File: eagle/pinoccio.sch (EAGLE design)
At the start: 48 parts, among them Q1 16MHz, Q2 32.768k, Q4 MOSFET-PCHANNEL, Q5 TRANSISTOR-NPN-DUAL, U1 MCP73831, U2 3.3V, U4 ATMEGA128RFA1, X1 USB-MICROB, Y2 ANTENNA2SMD5

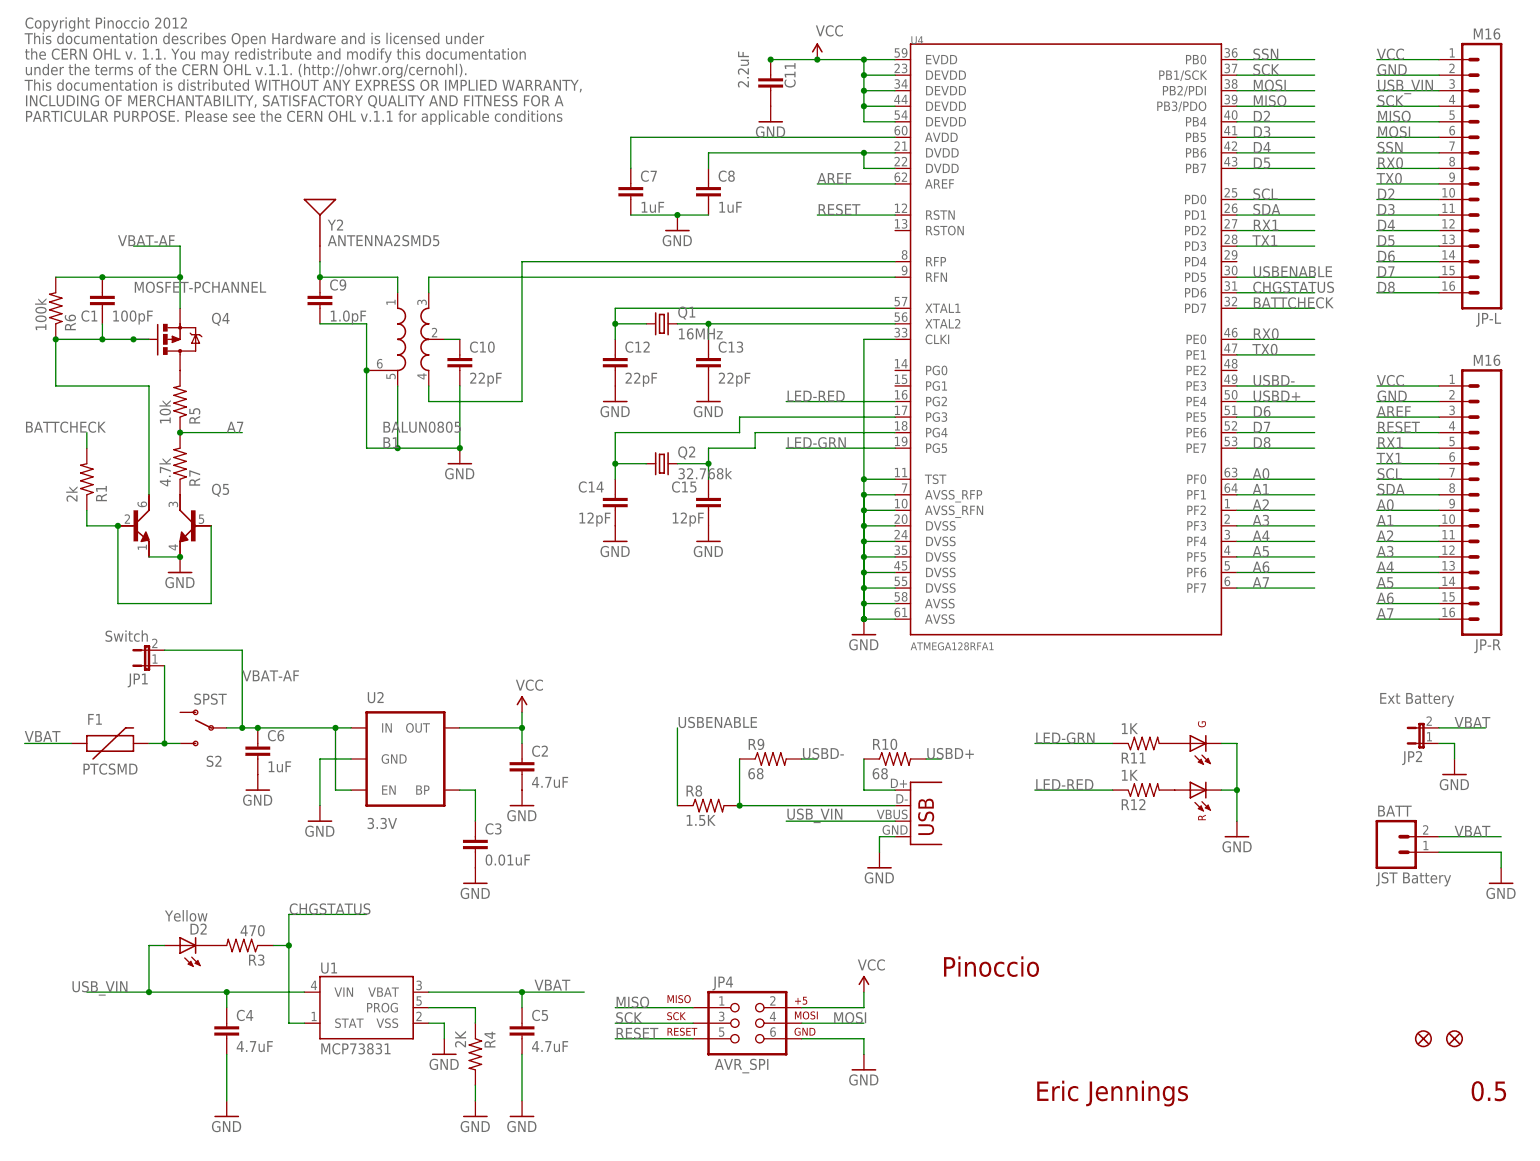
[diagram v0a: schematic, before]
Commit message: Version 0.6
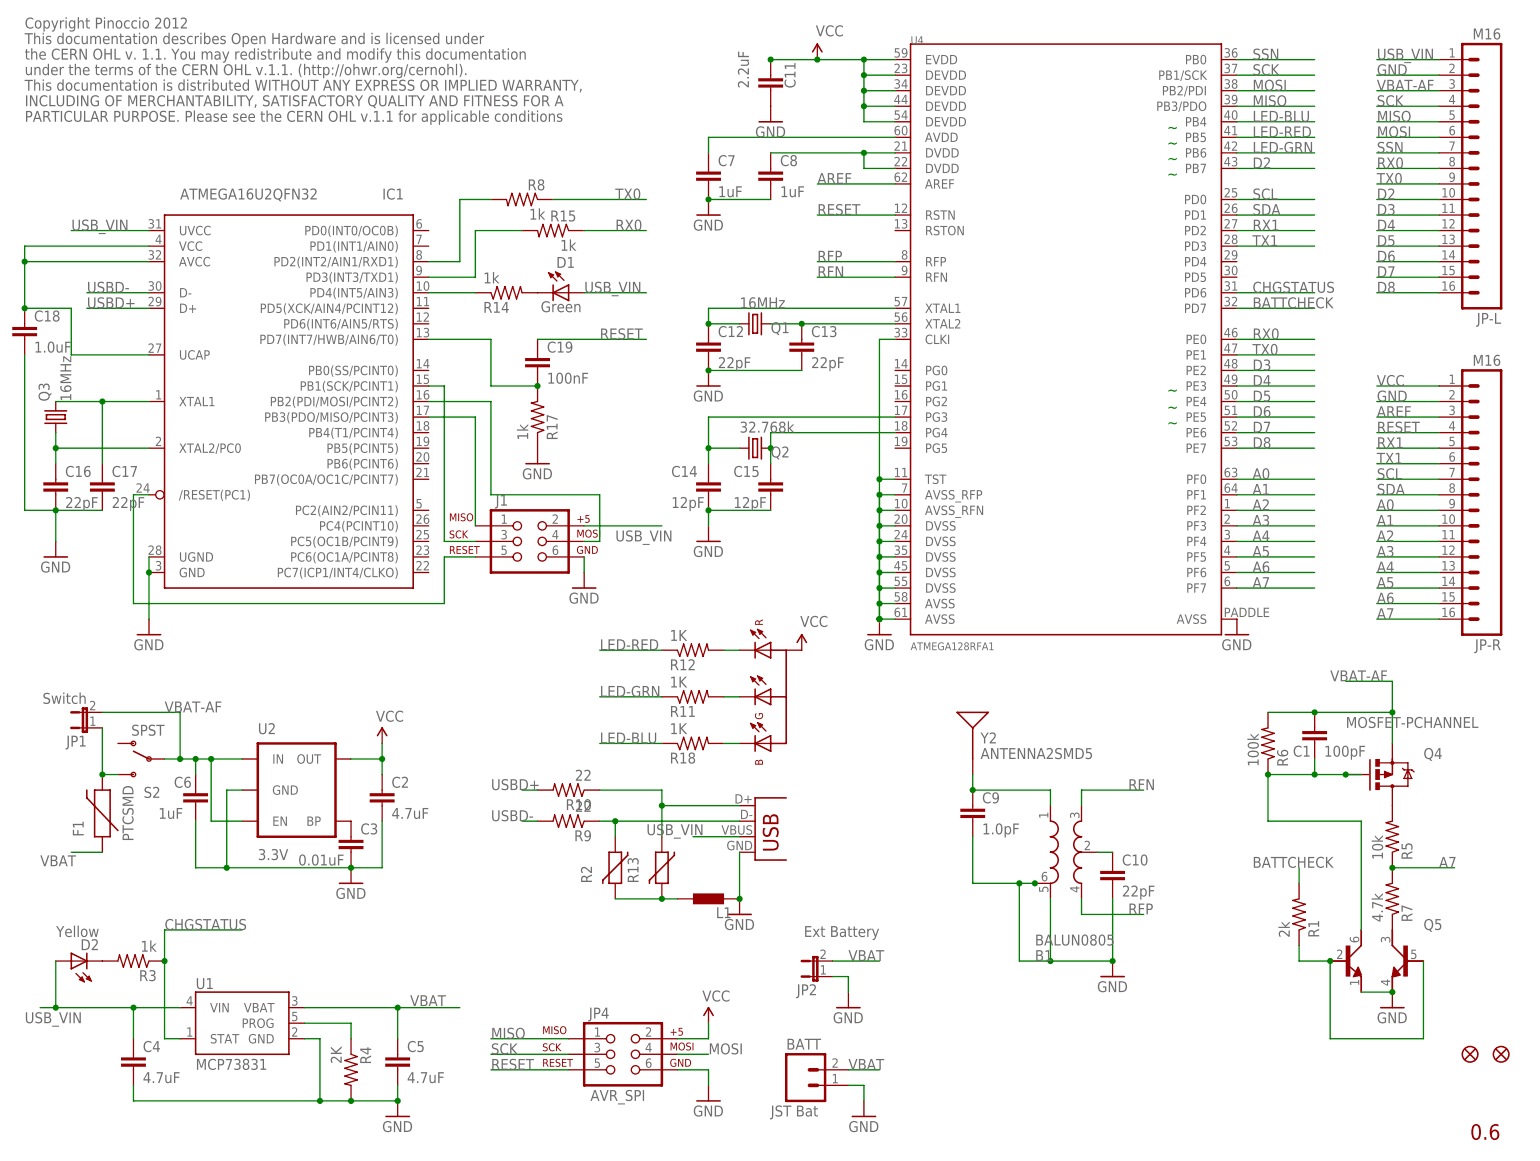
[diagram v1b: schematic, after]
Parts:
- removed U$4, U$5: FIDUCIAL1X2, SparkFun:FIDUCIAL1X2
- added C16, C17: 22pF, Pinoccio:CAP0402-CAP
- added C18: 1.0uF, Pinoccio:CAP0402-CAP
- added C19: 100nF, Pinoccio:CAP0402-CAP
- added D1: Green, Pinoccio:LED0603
- added IC1: ATMEGA16U2QFN32, Pinoccio:ATMEGA16U2QFN32
- added J1: AVR_SPI_PRG_6, Pinoccio:AVR_SPI_PRG_6
- added JP3, JP5: FIDUCIALUFIDUCIAL, Pinoccio:FIDUCIALUFIDUCIAL
- added L1: BML15H0603, Pinoccio:BML15H0603
- added Q3: 16MHz, BeanLabs:CRYSTALABM10
- added R13, R2: VARISTOR0402, Pinoccio:VARISTOR0402
- added R14, R15, R17: 1k, Pinoccio:RESISTOR0402-RES
- added R18: 1K, Pinoccio:RESISTOR0402-RES
- B1: device SparkFun:BALUN0805 -> Pinoccio:BALUN0805
- BATT: value JST Battery -> JST Bat
- C1, C10, C11, C12, C13, C14, C15, C2, C3, C4, C5, C6, C7, C8, C9: device SparkFun:CAP0402-CAP -> Pinoccio:CAP0402-CAP
- D2: device SparkFun:LED0603 -> Pinoccio:LED0603
- JP4: device SparkFun:AVR_SPI_PRG_6PTH -> Pinoccio:AVR_SPI_PRG_6PTH
- R1, R11, R12, R4, R5, R6, R7: device SparkFun:RESISTOR0402-RES -> Pinoccio:RESISTOR0402-RES
- R10, R9: value 68 -> 22; device SparkFun:RESISTOR0402-RES -> Pinoccio:RESISTOR0402-RES
- R3: value 470 -> 1k; device SparkFun:RESISTOR0402-RES -> Pinoccio:RESISTOR0402-RES
- R8: value 1.5K -> 1k; device SparkFun:RESISTOR0402-RES -> Pinoccio:RESISTOR0402-RES
- U$1: value LED-BICOLOR -> LED-RGBPLCC4; device Pinoccio:LED-BICOLOR -> Pinoccio:LED-RGBPLCC4
- U1: device SparkFun:MCP73831SMD -> Pinoccio:MCP73831
- X1: device SparkFun:USB-MICROB -> Pinoccio:USB-MICROB
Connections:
- net N$1 renamed RFN
- net N$52 renamed RFP
- removed net USBENABLE: R8.1, U4.PD5
- new net LED-BLU: R18.1, U4.PB4
- new net N$1: R12.2, U$1.R-C
- new net N$13: B1.RFGND@2, C10.1
- new net N$19: C16.1, IC1.XTAL2/PC0, Q3.1
- new net N$21: C17.1, IC1.XTAL1, Q3.2
- new net N$23: C18.1, IC1.AVCC, IC1.UCAP, IC1.VCC
- new net N$24: C19.2, IC1.PD7(INT7/HWB/AIN6/T0), R17.2
- new net N$55: IC1./RESET(PC1), J1.5
- new net N$56: IC1.PB3(PDO/MISO/PCINT3), J1.1
- new net N$57: IC1.PB2(PDI/MOSI/PCINT2), J1.4
- new net N$58: IC1.PB1(SCK/PCINT1), J1.3
- new net N$59: IC1.PD4(INT5/AIN3), R14.1
- new net N$62: D1.C, R14.2
- net D2: now also U4.PB7; no longer U4.PB4
- net D3: now also U4.PE2; no longer U4.PB5
- net D4: now also U4.PE3; no longer U4.PB6
- net D5: now also U4.PE4; no longer U4.PB7
- net GND: now also C16.2, C17.2, C18.2, IC1.GND, IC1.UGND, J1.6, L1.1, R17.1, U1.GND, U4.AVSS@PADDLE; no longer U$1.3, U$1.4, U1.VSS
- net LED-GRN: now also U4.PB6; no longer U4.PG5
- net LED-RED: now also U4.PB5; no longer U4.PG2
- net N$2: now also R2.1, R9.1, X1.D-; no longer B1.GND@2, C10.1
- net N$43: now also R13.1
- net N$5: now also U$1.G-C; no longer U$1.1
- net N$6: now also R18.2, U$1.B-C; no longer R12.2, U$1.2
- net N$9: now also L1.2, R13.2, R2.2; no longer R8.2, R9.1, X1.D-
- net RESET: now also C19.1
- net RX0: now also IC1.PD3(INT3/TXD1), R15.1, R15.2
- net TX0: now also IC1.PD2(INT2/AIN1/RXD1), R8.1, R8.2
- net USBD+: now also IC1.D+; no longer U4.PE4
- net USBD-: now also IC1.D-; no longer U4.PE3
- net USB_VIN: now also D1.A, IC1.UVCC, J1.2, JP-L.1; no longer JP-L.3
- net VBAT-AF: now also JP-L.3
- net VCC: now also U$1.A; no longer JP-L.1
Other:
- note added: "0.6"
- note added: "~"
- note removed: "0.5"
- note removed: "Eric Jennings"
- note removed: "Pinoccio"
- moved on the sheet: B1, BATT, C1, C10, C12, C13, C14, C15, C2, C3, C4, C5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

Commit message: Update to latest v0.6
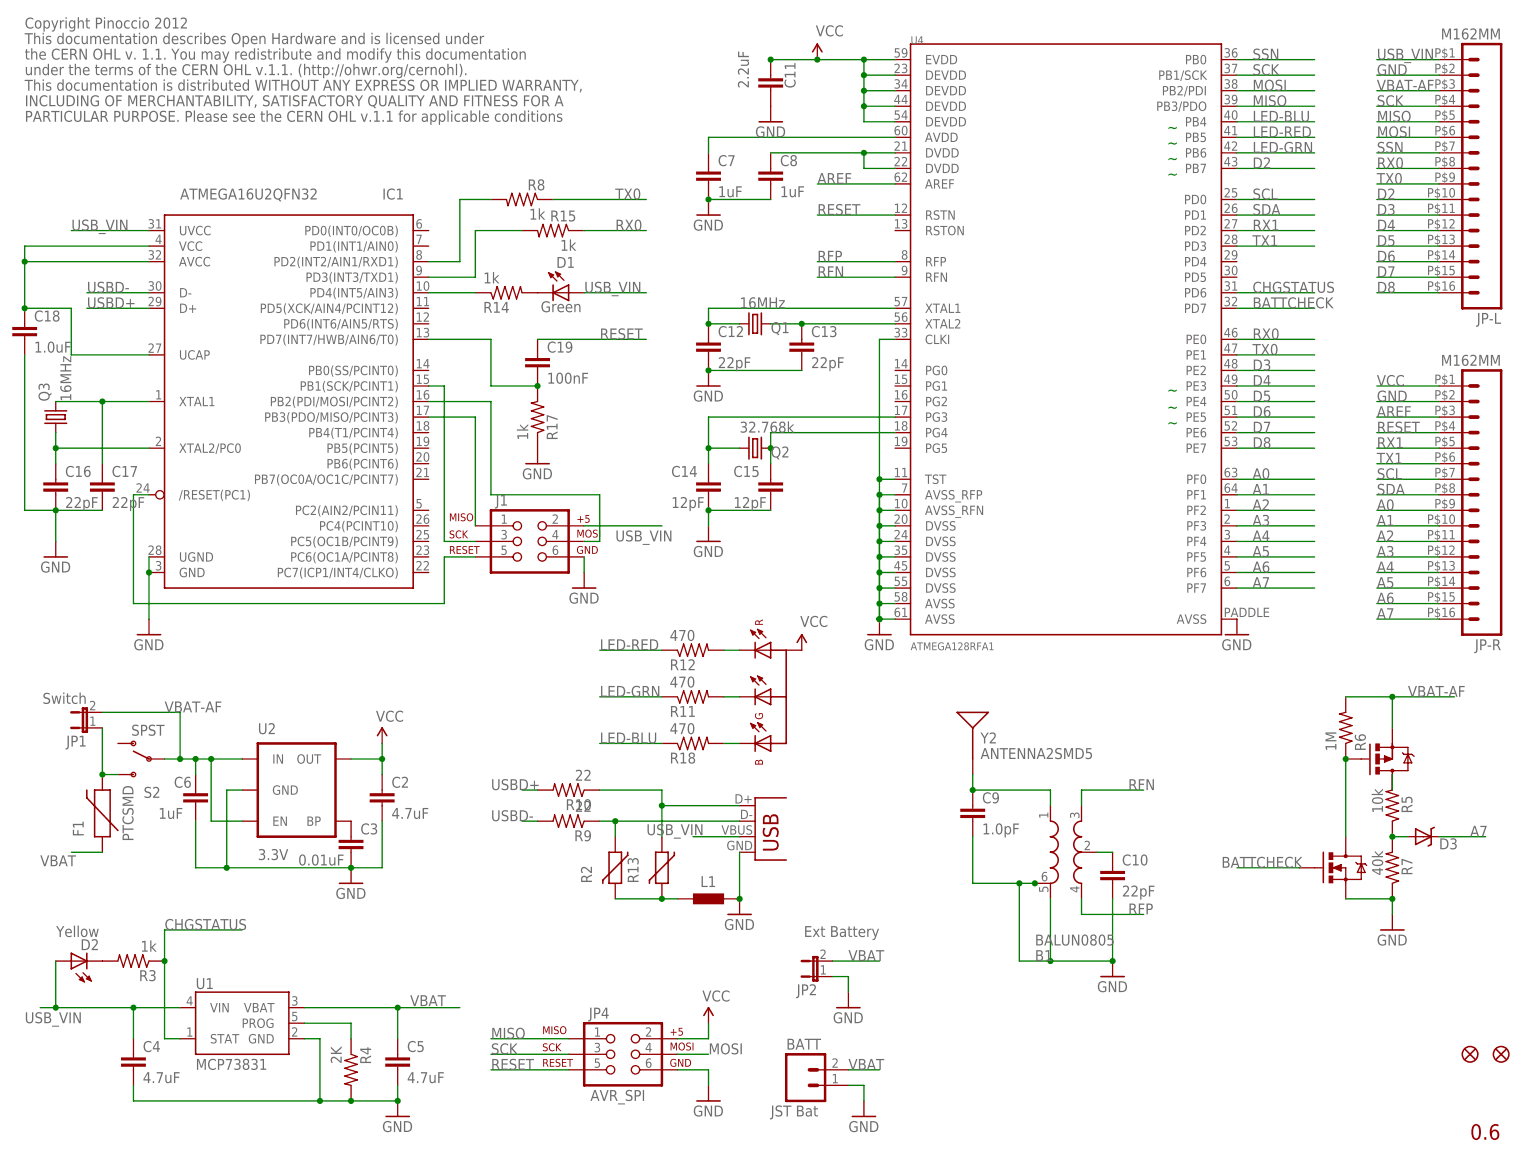
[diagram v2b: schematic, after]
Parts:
- removed C1: 100pF, Pinoccio:CAP0402-CAP
- removed Q4: MOSFET-PCHANNEL, Pinoccio:MOSFET-PCHANNELSMD
- removed Q5: TRANSISTOR-NPN-DUAL, Pinoccio:TRANSISTOR-NPN-DUAL
- removed R1: 2k, Pinoccio:RESISTOR0402-RES
- added D3: DIODE-SCHOTTKY, Pinoccio:DIODE-SCHOTTKY
- added U$2: MOSFET-DUAL-N-P, Pinoccio:MOSFET-DUAL-N-P
- JP-L, JP-R: value M16 -> M162MM; device SparkFun:M16 -> Pinoccio:M162MM
- R11, R12, R18: value 1K -> 470
- R6: value 100k -> 1M
- R7: value 4.7k -> 40k
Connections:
- removed net N$51: C1.2, Q4.G, Q5.1C, R6.1
- net A7: now also D3.C; no longer R5.1, R7.2
- net BATTCHECK: now also U$2G$N1.G; no longer R1.2
- net GND: now also R7.1, U$2G$N1.S; no longer Q5.1E, Q5.2E
- net N$14: now also D3.A, R5.1, R7.2; no longer Q5.2C, R7.1
- net N$3: now also U$2G$P2.D; no longer Q4.D
- net N$7: now also R6.1, U$2G$N1.D, U$2G$P2.G; no longer Q5.1B, Q5.2B, R1.1
- net VBAT-AF: now also U$2G$P2.S; no longer C1.1, Q4.S
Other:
- moved on the sheet: JP-L, JP-R, R5, R6, R7
